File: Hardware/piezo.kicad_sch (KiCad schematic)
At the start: 75 parts

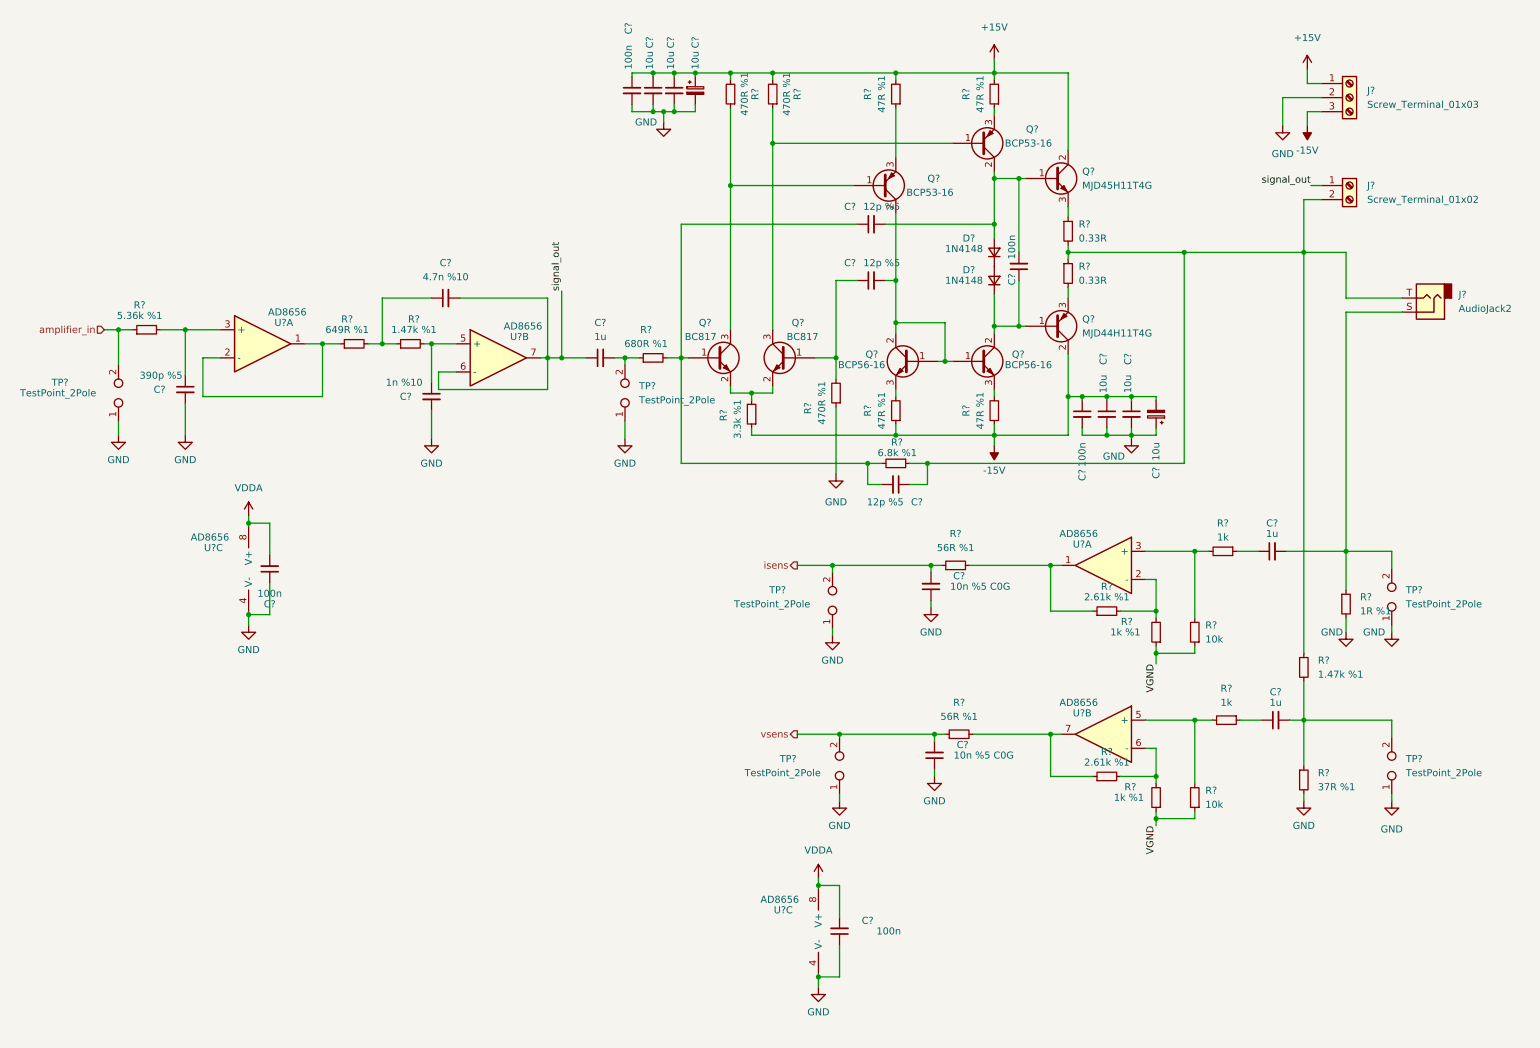
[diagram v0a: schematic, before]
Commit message: Completed schematic and PCB.
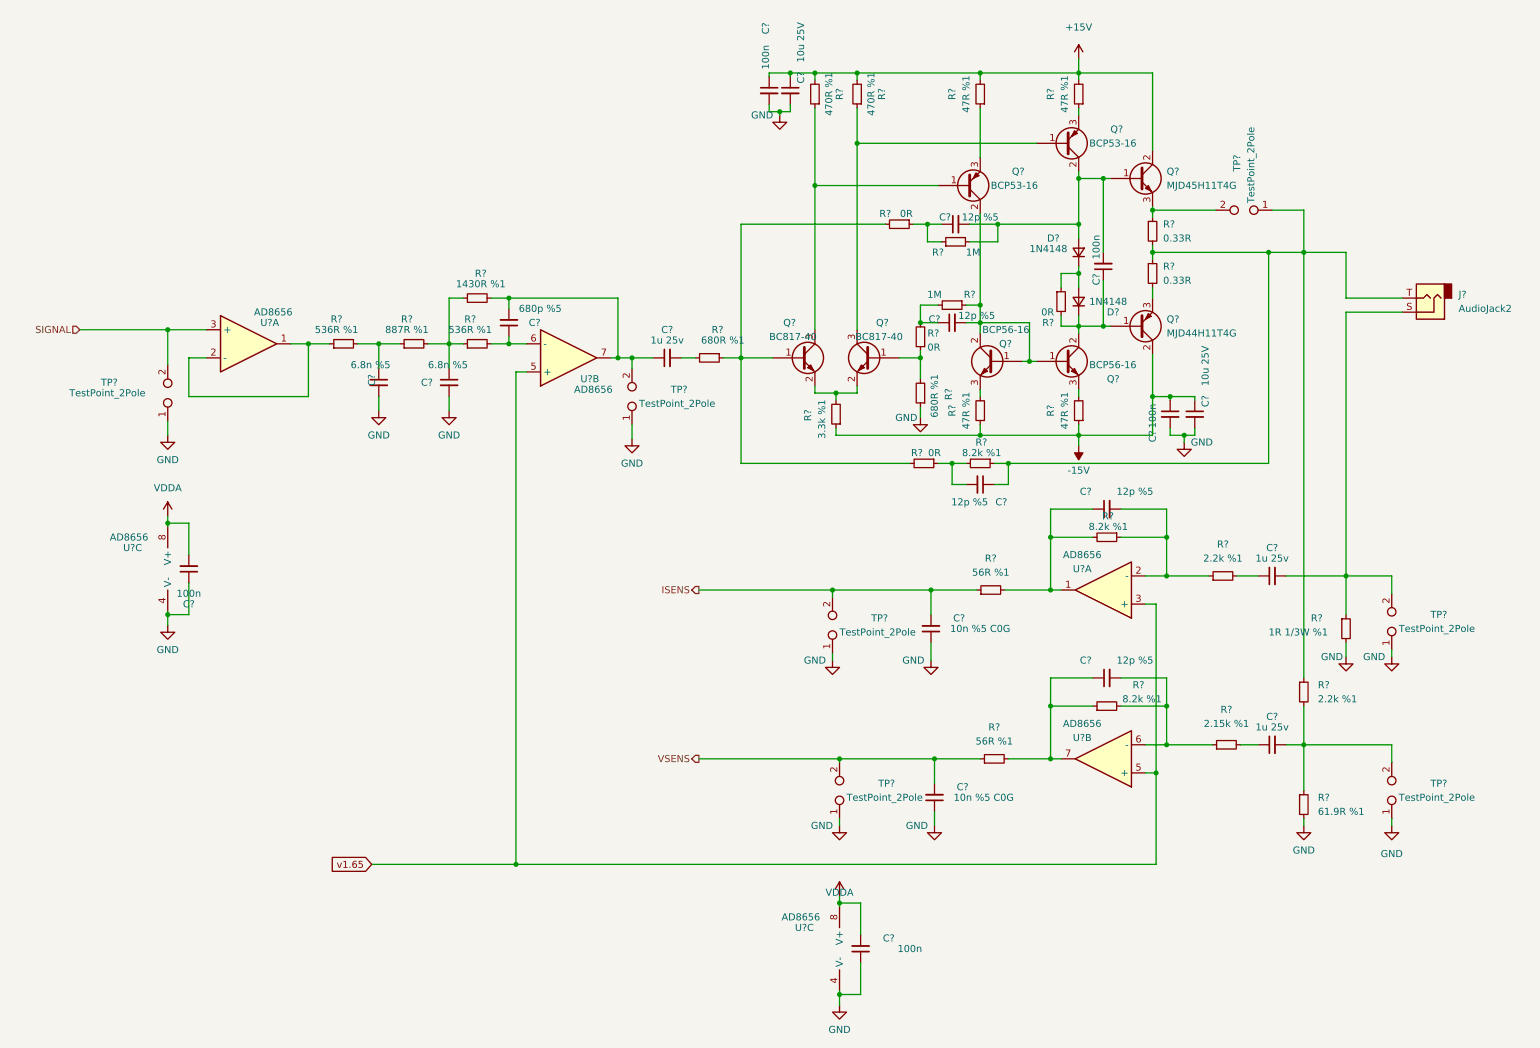
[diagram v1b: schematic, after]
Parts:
- removed C?: 4.7n %10, symbol Device:C_Small
- removed C? (x2): 12p %5, Capacitor_SMD:C_0603_1608Metric_Pad1.08x0.95mm_HandSolder, symbol Device:C_Small
- removed C?: 10n %5 C0G, Capacitor_SMD:C_0603_1608Metric_Pad1.08x0.95mm_HandSolder, symbol Device:C_Small
- removed C? (x4): 10u, symbol Device:C_Small
- removed C? (x3): 1u, symbol Device:C_Small
- removed C?: 390p %5, symbol Device:C_Small
- removed C?: 1n %10, symbol Device:C_Small
- removed C? (x2): 10u, symbol Device:C_Polarized_Small
- removed D?: 1N4148, symbol Device:D_Small
- removed J?: Screw_Terminal_01x03, symbol Connector:Screw_Terminal_01x03
- removed J?: Screw_Terminal_01x02, symbol Connector:Screw_Terminal_01x02
- removed Q? (x2): BCP53-16, Package_TO_SOT_SMD:SOT-223-3_TabPin2, symbol Transistor_BJT:BCP53
- removed Q? (x2): BC817, Package_TO_SOT_SMD:SOT-23, symbol Transistor_BJT:BC817
- removed R? (x2): 1k %1, symbol Device:R_Small
- removed R?: 5.36k %1, Resistor_SMD:R_0603_1608Metric_Pad0.98x0.95mm_HandSolder, symbol Device:R_Small
- removed R? (x2): 470R %1, Resistor_SMD:R_0603_1608Metric_Pad0.98x0.95mm_HandSolder, symbol Device:R_Small
- removed R? (x2): 2.61k %1, symbol Device:R_Small
- removed R? (x3): 47R %1, Resistor_SMD:R_0603_1608Metric_Pad0.98x0.95mm_HandSolder, symbol Device:R_Small
- removed R? (x2): 1k, symbol Device:R_Small
- removed R? (x2): 10k, symbol Device:R_Small
- removed R?: 1.47k %1, Resistor_SMD:R_0603_1608Metric_Pad0.98x0.95mm_HandSolder, symbol Device:R_Small
- removed R?: 680R %1, Resistor_SMD:R_0603_1608Metric_Pad0.98x0.95mm_HandSolder, symbol Device:R_Small
- removed R?: 56R %1, symbol Device:R_Small
- removed TP? (x5): TestPoint_2Pole, symbol Connector:TestPoint_2Pole
- removed U?: AD8656, Package_SO:SOIC-8_3.9x4.9mm_P1.27mm, symbol Device:Opamp_Dual
- added C? (x2): 6.8n %5, Capacitor_SMD:C_0805_2012Metric_Pad1.18x1.45mm_HandSolder, symbol Device:C_Small
- added C? (x3): 1u 25v, Capacitor_SMD:C_0603_1608Metric_Pad1.08x0.95mm_HandSolder, symbol Device:C_Small
- added C? (x4): 12p %5, Capacitor_SMD:C_0603_1608Metric_Pad1.08x0.95mm_HandSolder, symbol Device:C_Small
- added C? (x2): 10u 25V, Capacitor_SMD:C_1206_3216Metric_Pad1.33x1.80mm_HandSolder, symbol Device:C_Small
- added C?: 10n %5 C0G, Capacitor_SMD:C_0603_1608Metric_Pad1.08x0.95mm_HandSolder, symbol Device:C_Small
- added C?: 680p %5, Capacitor_SMD:C_0603_1608Metric_Pad1.08x0.95mm_HandSolder, symbol Device:C_Small
- added D?: 1N4148, Diode_SMD:D_SOD-123, symbol Device:D_Small
- added Q? (x2): BC817-40, Package_TO_SOT_SMD:SOT-23, symbol Transistor_BJT:BC817
- added Q? (x2): BCP53-16, Package_TO_SOT_SMD:SOT-223-3_TabPin2, symbol Transistor_BJT:BCP53
- added R? (x2): 536R %1, Resistor_SMD:R_0603_1608Metric_Pad0.98x0.95mm_HandSolder, symbol Device:R_Small
- added R?: 470R %1, Resistor_SMD:R_0603_1608Metric_Pad0.98x0.95mm_HandSolder, symbol Device:R_Small
- added R? (x4): 0R, symbol Device:R_Small
- added R? (x2): 1M, symbol Device:R_Small
- added R? (x2): 680R %1, Resistor_SMD:R_0603_1608Metric_Pad0.98x0.95mm_HandSolder, symbol Device:R_Small
- added R? (x2): 8.2k %1, Resistor_SMD:R_0603_1608Metric_Pad0.98x0.95mm_HandSolder, symbol Device:R_Small
- added R? (x3): 47R %1, Resistor_SMD:R_0603_1608Metric_Pad0.98x0.95mm_HandSolder, symbol Device:R_Small
- added R?: 2.2k %1, Resistor_SMD:R_0603_1608Metric_Pad0.98x0.95mm_HandSolder, symbol Device:R_Small
- added R?: 1430R %1, Resistor_SMD:R_0603_1608Metric_Pad0.98x0.95mm_HandSolder, symbol Device:R_Small
- added R?: 2.15k %1, Resistor_SMD:R_0603_1608Metric_Pad0.98x0.95mm_HandSolder, symbol Device:R_Small
- added R?: 56R %1, Resistor_SMD:R_0603_1608Metric_Pad0.98x0.95mm_HandSolder, symbol Device:R_Small
- added TP? (x6): TestPoint_2Pole, Connector_PinHeader_2.54mm:PinHeader_1x02_P2.54mm_Vertical, symbol Connector:TestPoint_2Pole
- added U?: AD8656, Package_SO:SOIC-8_3.9x4.9mm_P1.27mm, symbol Device:Opamp_Dual
- C? (x2): footprint (none) -> Capacitor_SMD:C_0603_1608Metric_Pad1.08x0.95mm_HandSolder; Link (none) -> https://ozdisan.com/passive-components/capacitors/smt-smd-a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
- C? (x2): Link (none) -> https://ozdisan.com/passive-components/capacitors/smt-smd-a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; Price (none) -> 0.00448
- D?: footprint (none) -> Diode_SMD:D_SOD-123; Link (none) -> https://ozdisan.com/power-semiconductors/diodes-diode-modul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; Price (none) -> 0.02794
- Q?: footprint (none) -> Package_TO_SOT_SMD:TO-252-2; Link (none) -> https://ozdisan.com/Product/Detail/448869/MJD44H11T4G; Price (none) -> 0.39273
- Q?: footprint (none) -> Package_TO_SOT_SMD:TO-252-2; Link (none) -> https://ozdisan.com/Product/Detail/448870/MJD45H11T4G; Price (none) -> 0.55649
- R?: value 6.8k %1 -> 8.2k %1; Link (none) -> https://ozdisan.com/passive-components/resistors/smt-smd-an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; Price (none) -> 0.00221
- R? (x3): Link (none) -> https://ozdisan.com/passive-components/resistors/smt-smd-an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; Price (none) -> 0.00221
- R?: value 649R %1 -> 887R %1; Link (none) -> https://ozdisan.com/passive-components/resistors/smt-smd-an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; Price (none) -> 0.00221
- R?: value 37R %1 -> 61.9R %1; footprint (none) -> Resistor_SMD:R_0603_1608Metric_Pad0.98x0.95mm_HandSolder; Link (none) -> https://ozdisan.com/passive-components/resistors/smt-smd-an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; Price (none) -> 0.00221
- R?: value 1.47k %1 -> 2.2k %1; footprint (none) -> Resistor_SMD:R_0603_1608Metric_Pad0.98x0.95mm_HandSolder; Link (none) -> https://ozdisan.com/passive-components/resistors/smt-smd-an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; Price (none) -> 0.00221
- R?: footprint (none) -> Resistor_SMD:R_0603_1608Metric_Pad0.98x0.95mm_HandSolder; Link (none) -> https://ozdisan.com/passive-components/resistors/smt-smd-an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; Price (none) -> 0.00221
- R?: value 1R %1 -> 1R 1/3W %1; footprint (none) -> Resistor_SMD:R_1210_3225Metric_Pad1.30x2.65mm_HandSolder; Link (none) -> https://ozdisan.com/passive-components/resistors/smt-smd-an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; Price (none) -> 0.05112
- TP?: footprint (none) -> Connector_PinHeader_2.54mm:PinHeader_1x02_P2.54mm_Vertical; Link (none) -> https://ozdisan.com/connectors-and-interconnects/headers/pi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; Price (none) -> 0.0091
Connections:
- net amplifier_in is gone; now on net SIGNAL: TP?.2
- net +15V: now also C?.1, R?.2, R?.2, R?.2
- net -15V: now also C?.1, R?.1
- net GND: now also C?.1, C?.2, C?.2, C?.2, C?.2, R?.1, TP?.1, TP?.1, TP?.1, TP?.1, TP?.1
- net at R?.2: now also C?.1, R?.1, R?.1
- net at R?.1: now also Q?.1 (B), Q?.3 (C)
- net at Q?.1 (B), Q?.1 (B), Q?.2 (C)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: now also C?.2, Q?.2 (C), Q?.4 (C), R?.1
- net at J?.S, R?.1: now also C?.2, TP?.2
- net at U?.1, U?.2 (-): now also R?.1; no longer R?.1
- net SIGNAL: now reaches U?.3 (+)
- net at J?.T, R?.1, R?.1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: now also C?.1, TP?.1
- net at R?.2: now also C?.2, R?.1; no longer C?.1
- net at R?.2: now also Q?.2 (E), Q?.2 (E)
- net at C?.1, Q?.1 (B), Q?.2 (C)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: now also D?.1 (K), R?.2
- net at R?.2: now also C?.1, R?.1, U?.7
- net at U?.2 (-): now also C?.2, R?.1, R?.1
- net at C?.2, C?.2, D?.2 (A)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: now also Q?.2 (C), Q?.4 (C), R?.2
- net at Q?.3 (E), R?.1: now also TP?.2
- net at U?.1: now also C?.1, R?.2, R?.2
- net v1.65: now reaches U?.3 (+)
- net v1.65: now also U?.5 (+), U?.5 (+)
- net at Q?.3 (E): now also R?.2
- net at R?.1, R?.2: now also C?.2, TP?.2
- net at D?.1 (K): now also D?.2 (A), R?.1
- net isens renamed ISENS
- net ISENS: now also R?.1, TP?.2
- net signal_out: no longer names the net of U?.6 (-)
- net signal_out: now also C?.1, R?.2; no longer U?.7
- net vsens renamed VSENS
- net VSENS: now also C?.2, TP?.2
- new net: Q?.1 (B), R?.1, R?.2, R?.2
- new net: Q?.1 (B), Q?.3 (C), R?.1
- new net: Q?.3 (E), R?.1 (x2)
- new net: C?.1, R?.2, R?.2
- new net: C?.1, R?.2 (x2)
- new net: C?.2, R?.2
- new net: C?.1, R?.1, R?.2
- new net: Q?.1 (B), R?.1, R?.2
- new net: C?.2, R?.1, R?.2, U?.6 (-)
- new net: C?.1, R?.1, R?.1
- new net: C?.1, C?.2, R?.2, TP?.2, U?.7
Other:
- moved on the sheet: C?, D?, Q?, R?, TP?, U?A, U?B, U?C
